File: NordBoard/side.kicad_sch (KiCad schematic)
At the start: 45 parts, among them SW1 SW_Push, SW15 SW_Push, SW16 SW_Push, SW2 SW_Push, SW22 SW_Push, SW23 SW_Push, SW24 SW_Push, SW25 SW_Push, SW26 SW_Push, SW27 SW_Push, SW28 SW_Push, SW29 SW_Push, SW3 SW_Push, SW30 SW_Push, SW31 SW_Push, SW32 SW_Push, SW33 SW_Push, SW34 SW_Push, SW4 SW_Push, SW9 SW_Push, U2 Seeeduino Xiao rp2040

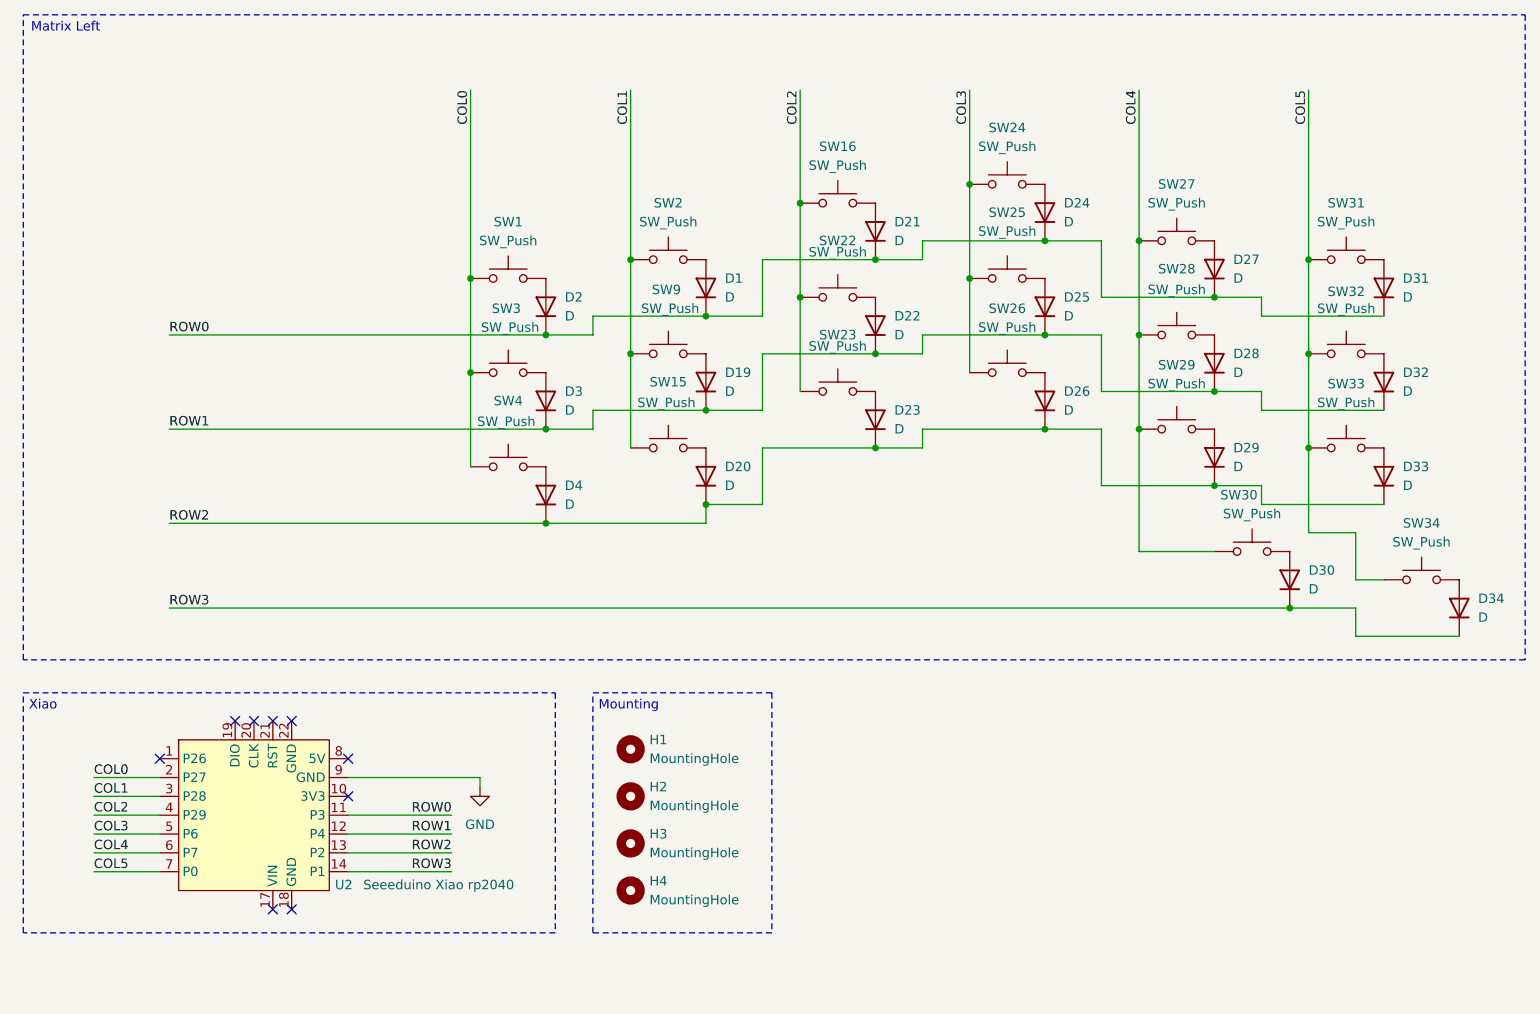
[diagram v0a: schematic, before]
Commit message: feat: revamp schem
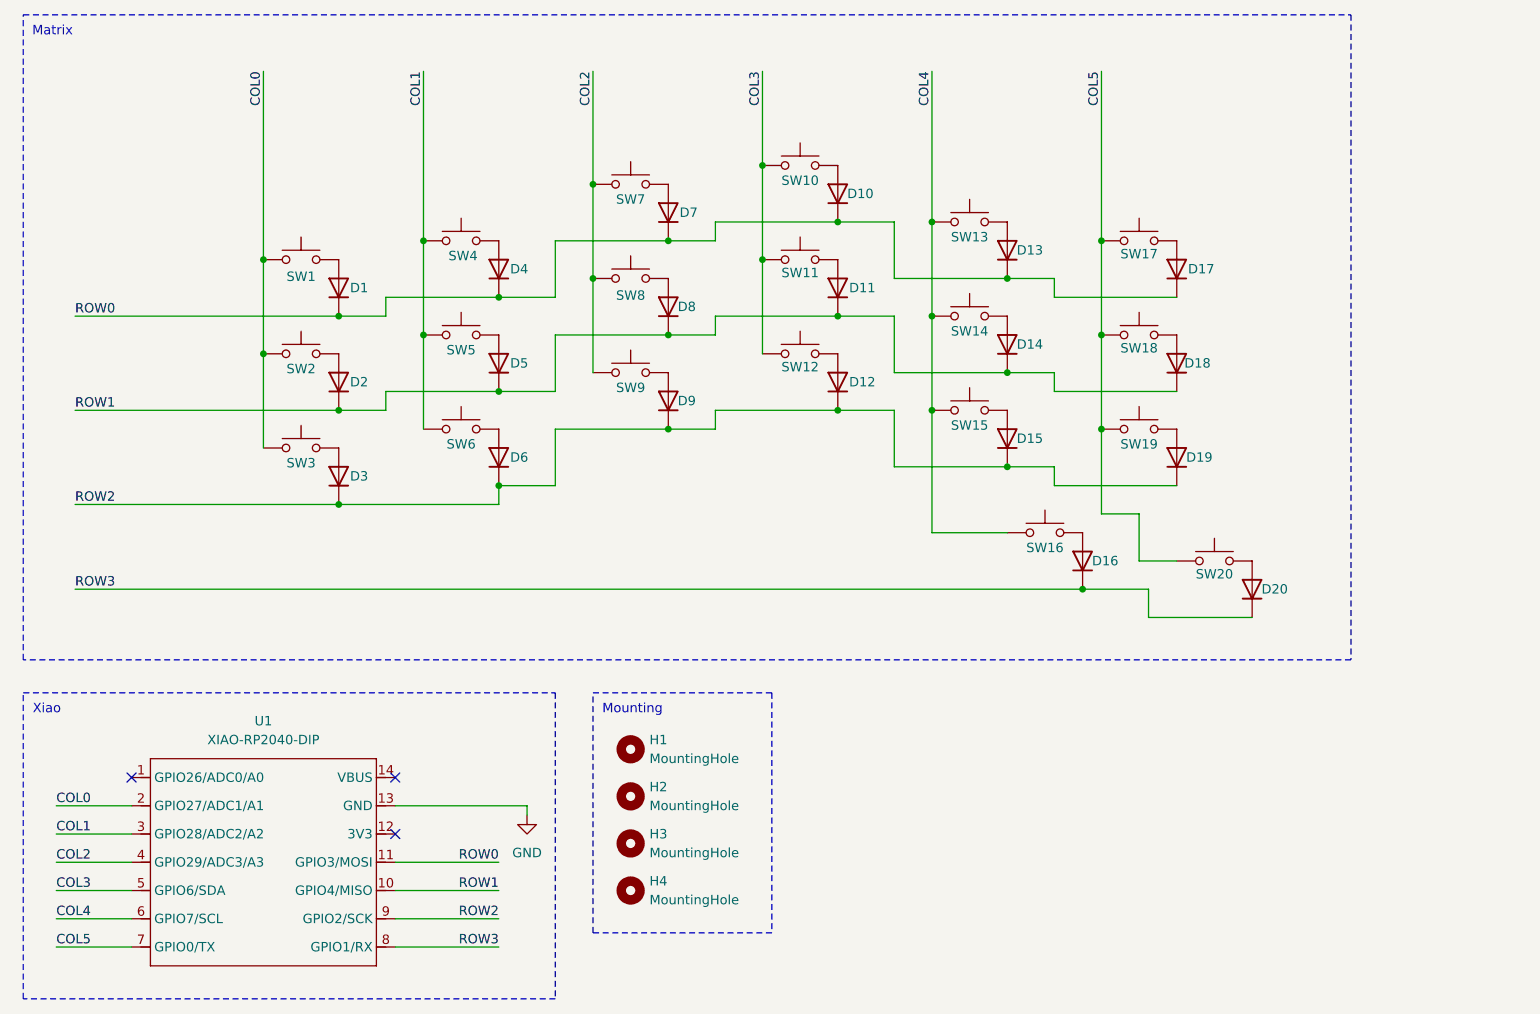
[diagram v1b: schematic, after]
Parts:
- removed U2: Seeeduino Xiao rp2040, PCM_marbastlib-xp-promicroish:Xiao_rp2040_ACH, symbol PCM_marbastlib-promicroish:Seeeduino_Xiao_rp2040
- added U1: XIAO-RP2040-DIP, Seeed Studio XIAO Series Library:XIAO-RP2040-DIP, symbol Seeed_Studio_XIAO_Series:XIAO-RP2040-DIP
- renumbered D2 to D1, D24 to D10, D25 to D11, D26 to D12, D27 to D13, D28 to D14, D29 to D15, D30 to D16, D31 to D17, D32 to D18, D33 to D19, D3 to D2, D34 to D20, D4 to D3, D1 to D4, D19 to D5, D20 to D6, D21 to D7, D22 to D8, D23 to D9, SW24 to SW10, SW25 to SW11, SW26 to SW12, SW27 to SW13, SW28 to SW14, SW29 to SW15, SW30 to SW16, SW31 to SW17, SW32 to SW18, SW33 to SW19, SW3 to SW2, SW34 to SW20, SW4 to SW3, SW2 to SW4, SW9 to SW5, SW15 to SW6, SW16 to SW7, SW22 to SW8, SW23 to SW9
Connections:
- net COL0: now also U1.2 (GPIO27/ADC1/A1)
- net COL1: now also U1.3 (GPIO28/ADC2/A2)
- net COL2: now also U1.4 (GPIO29/ADC3/A3)
- net COL3: now also U1.5 (GPIO6/SDA)
- net COL4: now also U1.6 (GPIO7/SCL)
- net COL5: now also U1.7 (GPIO0/TX)
- net GND: now also U1.13 (GND)
- net ROW0: now also U1.11 (GPIO3/MOSI)
- net ROW1: now also U1.10 (GPIO4/MISO)
- net ROW2: now also U1.9 (GPIO2/SCK)
- net ROW3: now also U1.8 (GPIO1/RX)
- no-connect marks 9 -> 3
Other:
- note added: "Matrix"
- note removed: "Matrix Left"
- moved on the sheet: D1, D10, D11, D12, D13, D14, D15, D16, D17, D18, D19, D2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

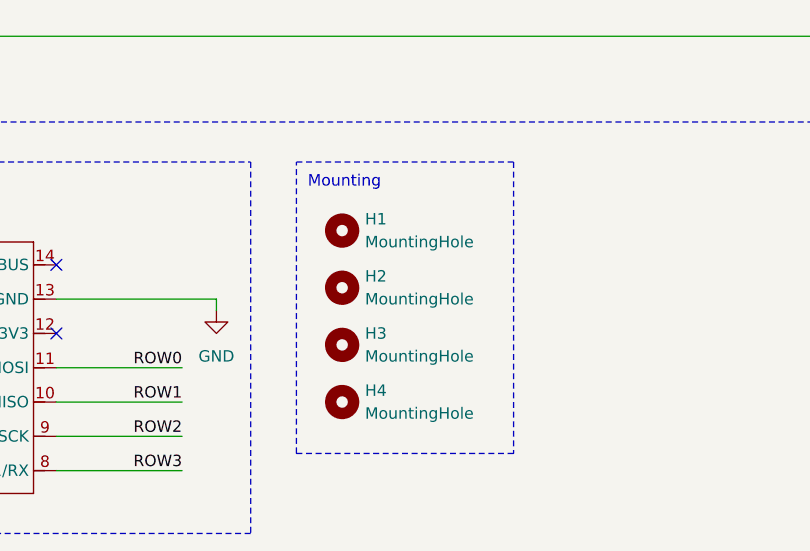
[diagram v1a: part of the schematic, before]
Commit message: chore: pcb board cleanup
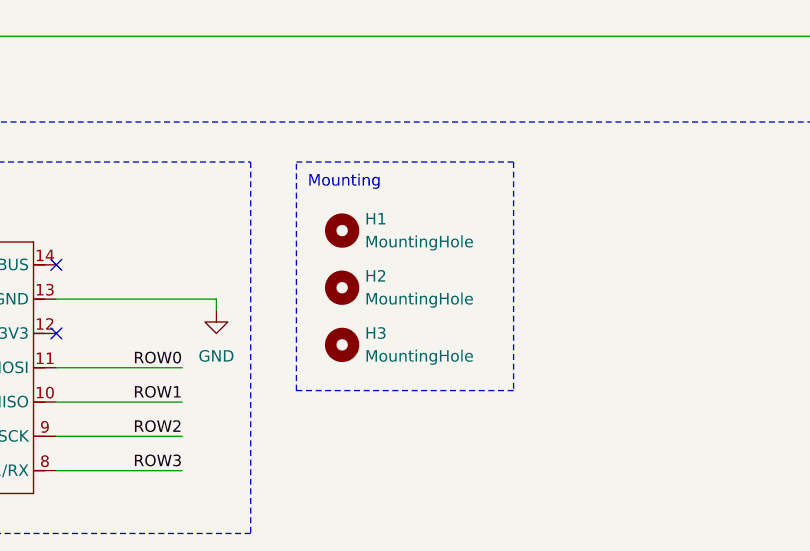
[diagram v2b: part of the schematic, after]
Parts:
- removed H4: MountingHole, MountingHole:MountingHole_2.2mm_M2, symbol Mechanical:MountingHole
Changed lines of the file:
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@@
 	(rectangle
 		(start 101.6 110.49)
-		(end 125.73 142.875)
+		(end 125.73 135.89)
 		(stroke
 			(width 0)
@@
 				)
 				(path "/7cf7f72d-7ab1-4807-b592-339093d5ca44/a5832e99-b0f3-4441-a24d-2a862f25015f"
-					(reference "H5")
+					(reference "H4")
 					(unit 1)
 				)
@@
 	)
 	(symbol
-		(lib_id "Mechanical:MountingHole")
-		(at 106.68 137.16 0)
-		(unit 1)
-		(exclude_from_sim no)
-		(in_bom no)
-		(on_board yes)
-		(dnp no)
-		(fields_autoplaced yes)
-		(property "Reference" "H4"
-			(at 109.22 135.8899 0)
-			(effects
-				(font
-					(size 1.27 1.27)
-				)
-				(justify left)
-			)
-		)
-		(property "Value" "MountingHole"
-			(at 109.22 138.4299 0)
-			(effects
-				(font
-					(size 1.27 1.27)
-				)
-				(justify left)
-			)
-		)
-		(property "Footprint" "MountingHole:MountingHole_2.2mm_M2"
-			(at 106.68 137.16 0)
-			(effects
-				(font
-					(size 1.27 1.27)
-				)
-				(hide yes)
-			)
-		)
-		(property "Datasheet" "~"
-			(at 106.68 137.16 0)
-			(effects
-				(font
-					(size 1.27 1.27)
-				)
-				(hide yes)
-			)
-		)
-		(property "Description" "Mounting Hole without connection"
-			(at 106.68 137.16 0)
-			(effects
-				(font
-					(size 1.27 1.27)
-				)
-				(hide yes)
-			)
-		)
-		(instances
-			(project "NordBoard"
-				(path "/7cf7f72d-7ab1-4807-b592-339093d5ca44/7e48f610-41a3-4552-82fa-dd005ce074be"
-					(reference "H4")
-					(unit 1)
-				)
-				(path "/7cf7f72d-7ab1-4807-b592-339093d5ca44/a5832e99-b0f3-4441-a24d-2a862f25015f"
-					(reference "H8")
-					(unit 1)
-				)
-			)
-		)
-	)
-	(symbol
 		(lib_id "Switch:SW_Push")
 		(at 162.56 88.9 0)
@@
 				)
 				(path "/7cf7f72d-7ab1-4807-b592-339093d5ca44/a5832e99-b0f3-4441-a24d-2a862f25015f"
-					(reference "H6")
+					(reference "H5")
 					(unit 1)
 				)
@@
 				)
 				(path "/7cf7f72d-7ab1-4807-b592-339093d5ca44/a5832e99-b0f3-4441-a24d-2a862f25015f"
-					(reference "H7")
+					(reference "H6")
 					(unit 1)
 				)
